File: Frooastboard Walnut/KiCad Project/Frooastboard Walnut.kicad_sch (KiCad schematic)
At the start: 172 parts, among them SW1 SW_Push, U1 ATmega32U4-A, Y1 Crystal_GND24_Small

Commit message: rotate iso enter switch
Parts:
- KEY_ENTER1: footprint MX_Only:MXOnly-ISO-NoLED-NoStabilizers -> MX_Only:MXOnly-ISO-ROTATED-NoLED-NoStabilizers
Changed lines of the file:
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@@
       (effects (font (size 0.508 0.508)))
     )
-    (property "Footprint" "MX_Only:MXOnly-ISO-NoLED-NoStabilizers" (id 2) (at 113.665 131.445 0)
+    (property "Footprint" "MX_Only:MXOnly-ISO-ROTATED-NoLED-NoStabilizers" (id 2) (at 113.665 131.445 0)
       (effects (font (size 1.524 1.524)) hide)
     )
@@
     )
     (path "/53c8ac3c-456e-47c9-a6eb-2ee6377474f4"
-      (reference "KEY_ENTER1") (unit 1) (value "MX-NoLED") (footprint "MX_Only:MXOnly-ISO-NoLED-NoStabilizers")
+      (reference "KEY_ENTER1") (unit 1) (value "MX-NoLED") (footprint "MX_Only:MXOnly-ISO-ROTATED-NoLED-NoStabilizers")
     )
     (path "/fbda3cca-a5fe-4f20-8515-486859fc314e"

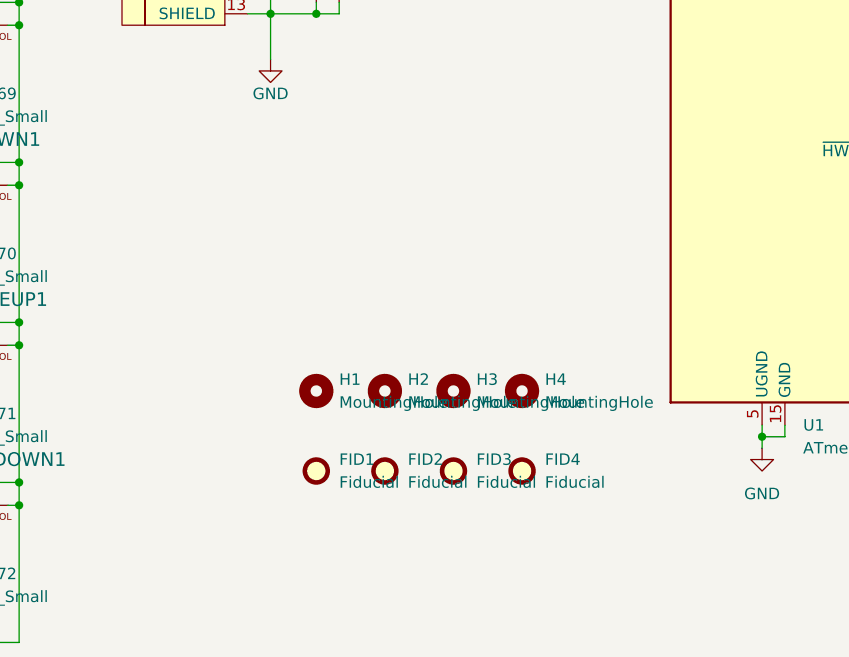
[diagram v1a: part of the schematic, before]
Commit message: Mounting Holes
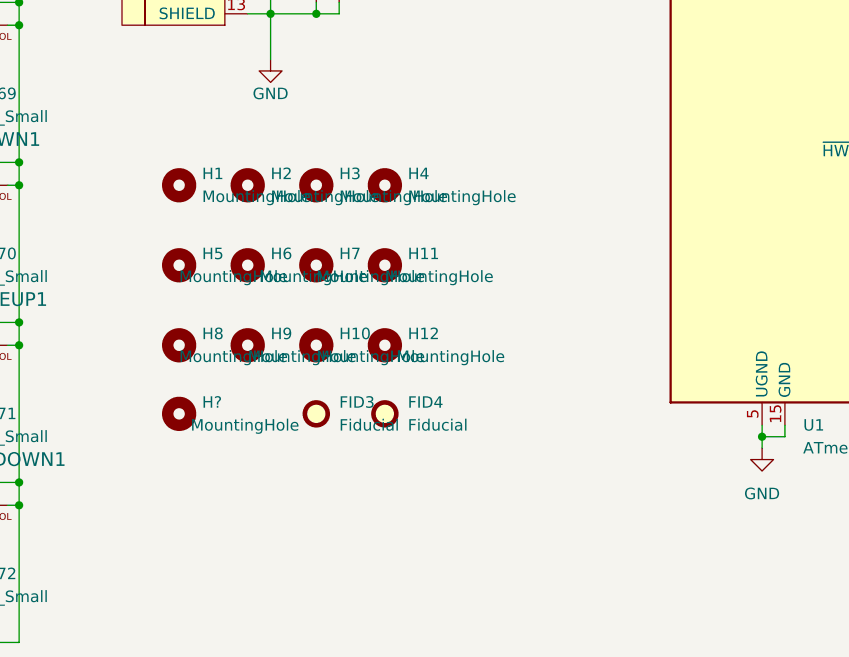
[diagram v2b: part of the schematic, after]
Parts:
- removed FID1, FID2: Fiducial, Fiducial:Fiducial_1mm_Mask2mm, symbol Mechanical:Fiducial
- added H10, H11, H12, H5, H6, H7, H8, H9, H?: MountingHole, MountingHole:MountingHole_3.2mm_M3_DIN965, symbol Mechanical:MountingHole
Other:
- moved on the sheet: FID3, FID4, H1, H2, H3, H4
